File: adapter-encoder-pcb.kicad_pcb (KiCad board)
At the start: 2 copper layers, 12 x 12 mm, 21 parts, among them IC1 THVD2410VDRCR, M1 THRU_HOLE_PAD, M2 THRU_HOLE_PAD, U1 TLE5009E1000FUMA1, U2 STM32L011F4Ux, U3 DF52-4S-0.8H(21), U4 SPX3819M5-L-3-3

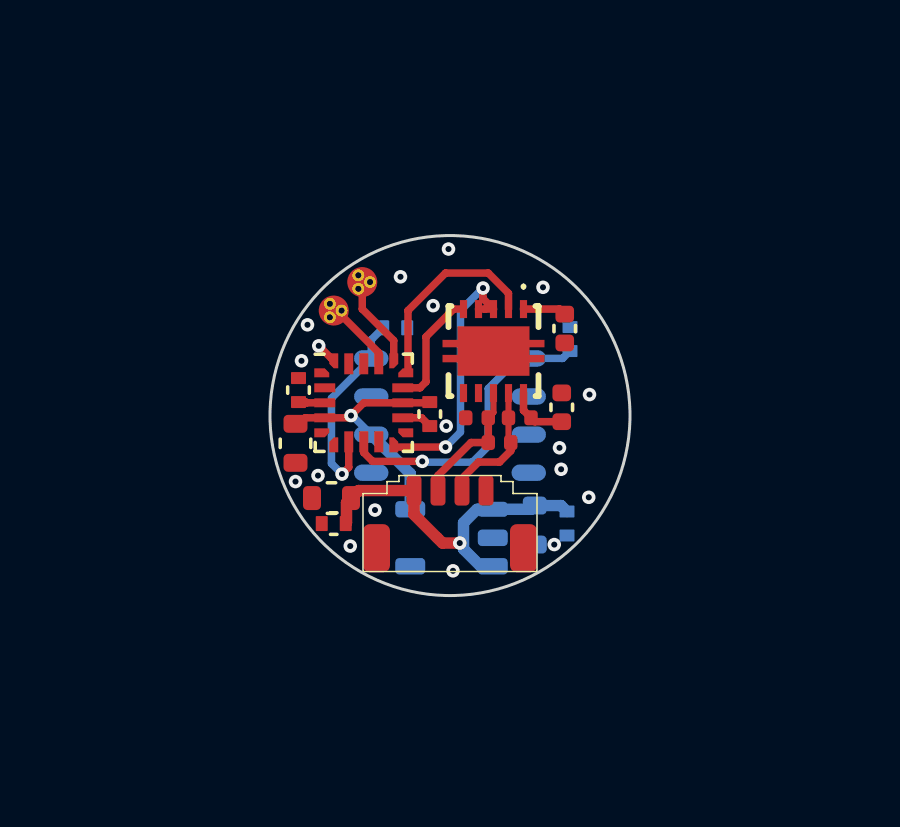
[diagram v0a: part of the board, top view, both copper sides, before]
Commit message: mostly routed updated board
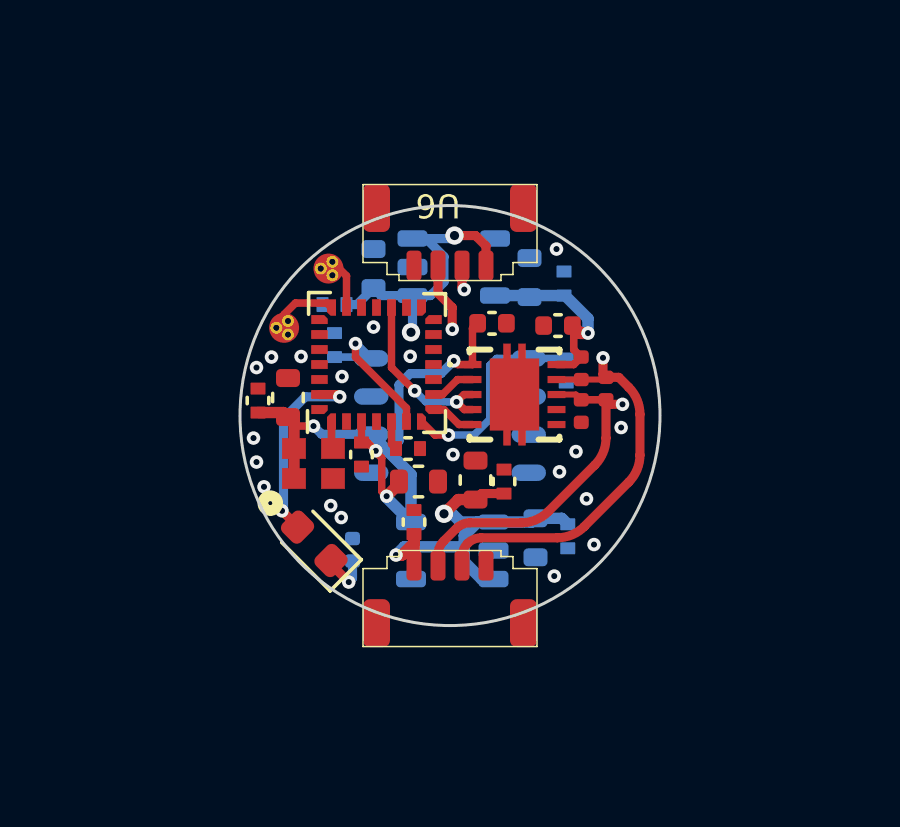
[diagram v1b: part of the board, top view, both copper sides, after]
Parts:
- added C12: 4.7uF, adapter-encoder:C_0603_1608Metric, F.Cu at (139.5, 111.0)
- added C13: 100nF, adapter-encoder:C_0402_1005Metric, F.Cu at (138.5, 111.1)
- added C14: 100nF, adapter-encoder:C_0402_1005Metric, B.Cu at (141.1, 107.9)
- added C15: 4.7uF, adapter-encoder:C_0603_1608Metric, B.Cu at (142.4, 106.7)
- added C16: 100nF, adapter-encoder:C_0402_1005Metric, B.Cu at (148.7, 107.2)
- added C17: 4.7uF, adapter-encoder:C_0603_1608Metric, B.Cu at (147.6, 107.0)
- added C18: 100nF, adapter-encoder:C_0402_1005Metric, F.Cu at (146.7, 113.8)
- added D1: LED, adapter-encoder:LED_0603_1608Metric, F.Cu at (140.4, 115.9)
- added R1: Resistor, adapter-encoder:R_0402_1005Metric, B.Cu at (141.7, 116.1)
- added U5: C2901617, adapter-encoder:ECS-1633-480-BN-TR, F.Cu at (140.4, 113.2)
- added U6: DF52-4S-0.8H(21), adapter-encoder:DF52-4S-0.8H(21), F.Cu at (144.9, 106.6)
- added U7: SPX3819M5-L-3-3, adapter-encoder:SOT-23-5, B.Cu at (145.0, 106.7)
- U2: value STM32L011F4Ux -> STM32G031G6U6; footprint adapter-encoder:ST_UFQFPN-20_3x3mm_P0.5mm -> adapter-encoder:UFQFPN28
- moved C8 4.84 mm to (145.8, 113.8), turned to 90 degrees
- moved C1 4.29 mm to (143.9, 113.8), turned to 0 degrees
- moved C5 4.14 mm to (143.5, 112.7), turned to 0 degrees
- moved R3 3.98 mm to (150.1, 110.7), turned to 90 degrees
- moved R4 3.48 mm to (149.3, 111.5), turned to 90 degrees
- moved M1 3.02 mm to (139.4, 108.7), turned to 90 degrees
- moved C7 2.73 mm to (148.5, 108.6), turned to 0 degrees
- moved C11 2.68 mm to (143.7, 115.2), turned to 90 degrees
- moved C3 2.65 mm to (142.0, 112.9)
- moved R2 2.63 mm to (149.3, 110.1), turned to 90 degrees
- moved U3 2.50 mm to (144.9, 116.6)
- moved C6 2.43 mm to (146.3, 108.6), turned to 180 degrees
- moved C4 2.11 mm to (141.1, 109.3), turned to 90 degrees
- moved IC1 1.61 mm to (147.1, 110.9), turned to 0 degrees
- moved M2 1.41 mm to (140.9, 106.7), turned to 90 degrees
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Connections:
- C1 pad 1: /3v3 -> +3V3
- C3 pad 1: /3v3 -> +3V3
- C5 pad 1: Net-(U2-NRST) -> Net-(U2-PF2-NRST)
- U1 pad 6: /3v3 -> +3V3
- U2 pad 1: unconnected-(U2-PC14-Pad1) -> Net-(U2-PC14-OSC32_IN)
- U2 pad 10: /UART1_DE -> unconnected-(U2-PA4-Pad10)
- U2 pad 11: /LED_GPIO -> unconnected-(U2-PA5-Pad11)
- U2 pad 12: GND -> unconnected-(U2-PA6-Pad12)
- U2 pad 13: /3v3 -> unconnected-(U2-PA7-Pad13)
- U2 pad 14: /TX -> unconnected-(U2-PB0-Pad14)
- U2 pad 15: /RX -> unconnected-(U2-PB1-Pad15)
- U2 pad 16: /SWDIO -> unconnected-(U2-PA8-Pad16)
- U2 pad 17: /SWCLK -> /UART1_DE
- U2 pad 20: GND -> /SWCLK
- U2 pad 3: Net-(U2-NRST) -> +3V3
- U2 pad 4: /3v3 -> GND
- U2 pad 5: /V_TEMP -> Net-(U2-PF2-NRST)
- U2 pad 6: unconnected-(U2-PA1-Pad6) -> /SIN
- U2 pad 7: /SIN -> /COS
- U2 pad 8: /COS -> /TX
- U2 pad 9: unconnected-(U2-PA6-Pad9) -> /RX
- U4 pad 5: /3v3 -> +3V3
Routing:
- net /Vin: track 11.7 -> 35.8 mm, vias 1 -> 4
- net +3V3: track 1.45 -> 22.6 mm, vias 0 -> 4
- net /B-PROTECTED: track 4.36 -> 21.1 mm, vias 0 -> 2
- net /A-PROTECTED: track 4.35 -> 20.6 mm, vias 0 -> 2
- net /3v3: track 8.76 -> 0.00 mm, vias 1 -> 0
- net /LED_GPIO: track 0.00 -> 6.73 mm, vias 0 -> 2
- net /RX: track 6.75 -> 1.51 mm
- net /+5V0: track 2.01 -> 6.63 mm, vias 0 -> 1
- net /UART1_DE: track 8.89 -> 5.91 mm
- net /COS: track 10.0 -> 7.13 mm
- net /TX: track 3.99 -> 1.51 mm
- net Net-(D1-K): track 0.00 -> 1.72 mm, vias 0 -> 1
- net GND: track 1.69 -> 0.00 mm, vias 18 -> 19
- net /SIN: track 6.90 -> 5.28 mm
- net Net-(U2-PF2-NRST): track 0.00 -> 0.96 mm
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- added copper zone on In1.Cu, net GND
- added copper zone on In2.Cu, net GND
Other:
- board size 12 x 12 mm -> 14 x 14 mm
- copper layers 2 -> 4
